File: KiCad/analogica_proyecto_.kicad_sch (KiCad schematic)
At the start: 4 parts, among them U2 ACS714xLCTR-50A, U3 ACS714xLCTR-50A

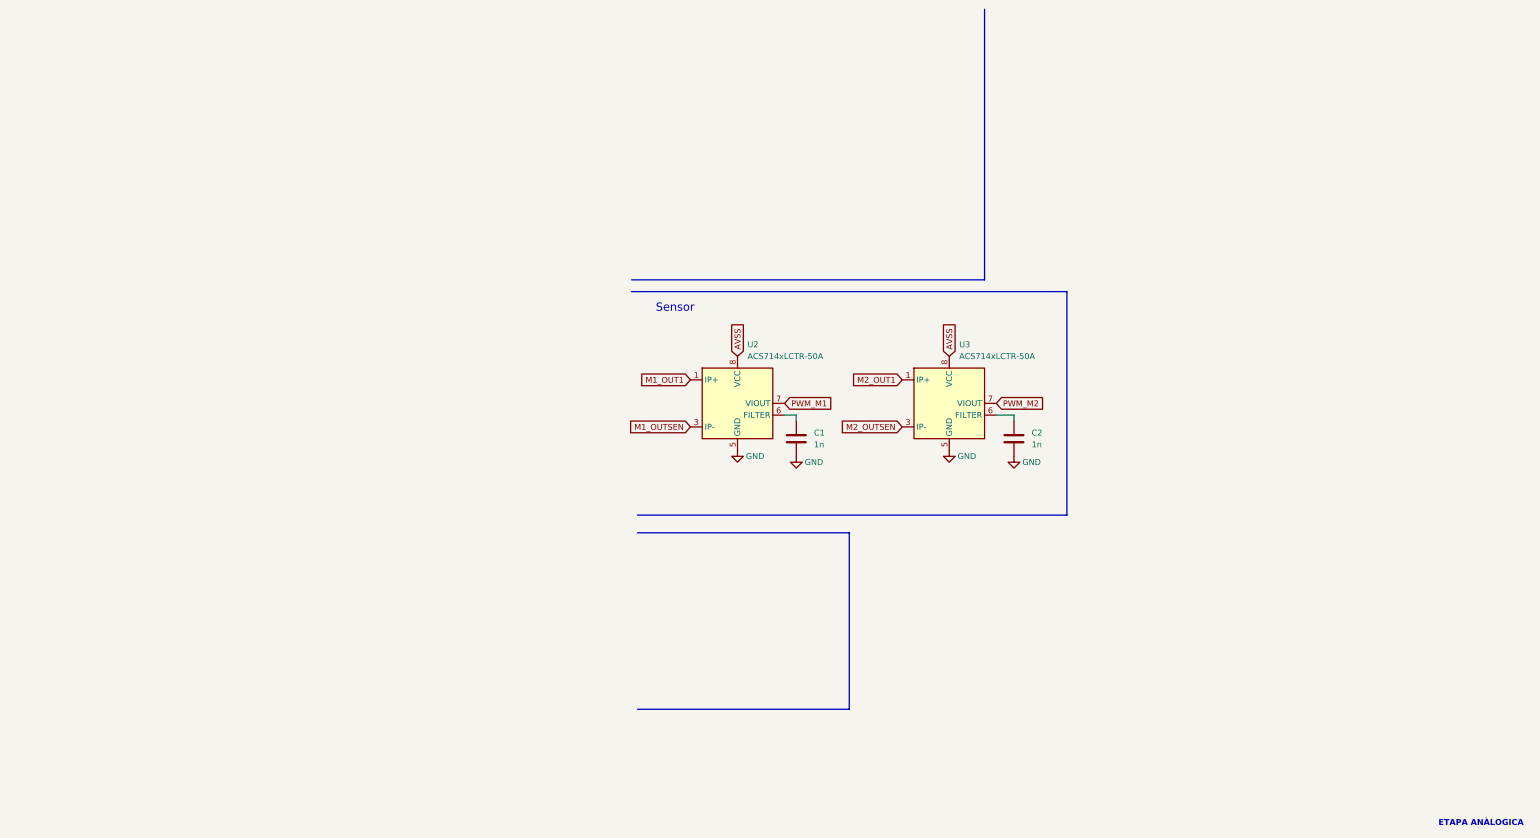
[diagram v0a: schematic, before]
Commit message: Nuevos cambios esquemativo v3
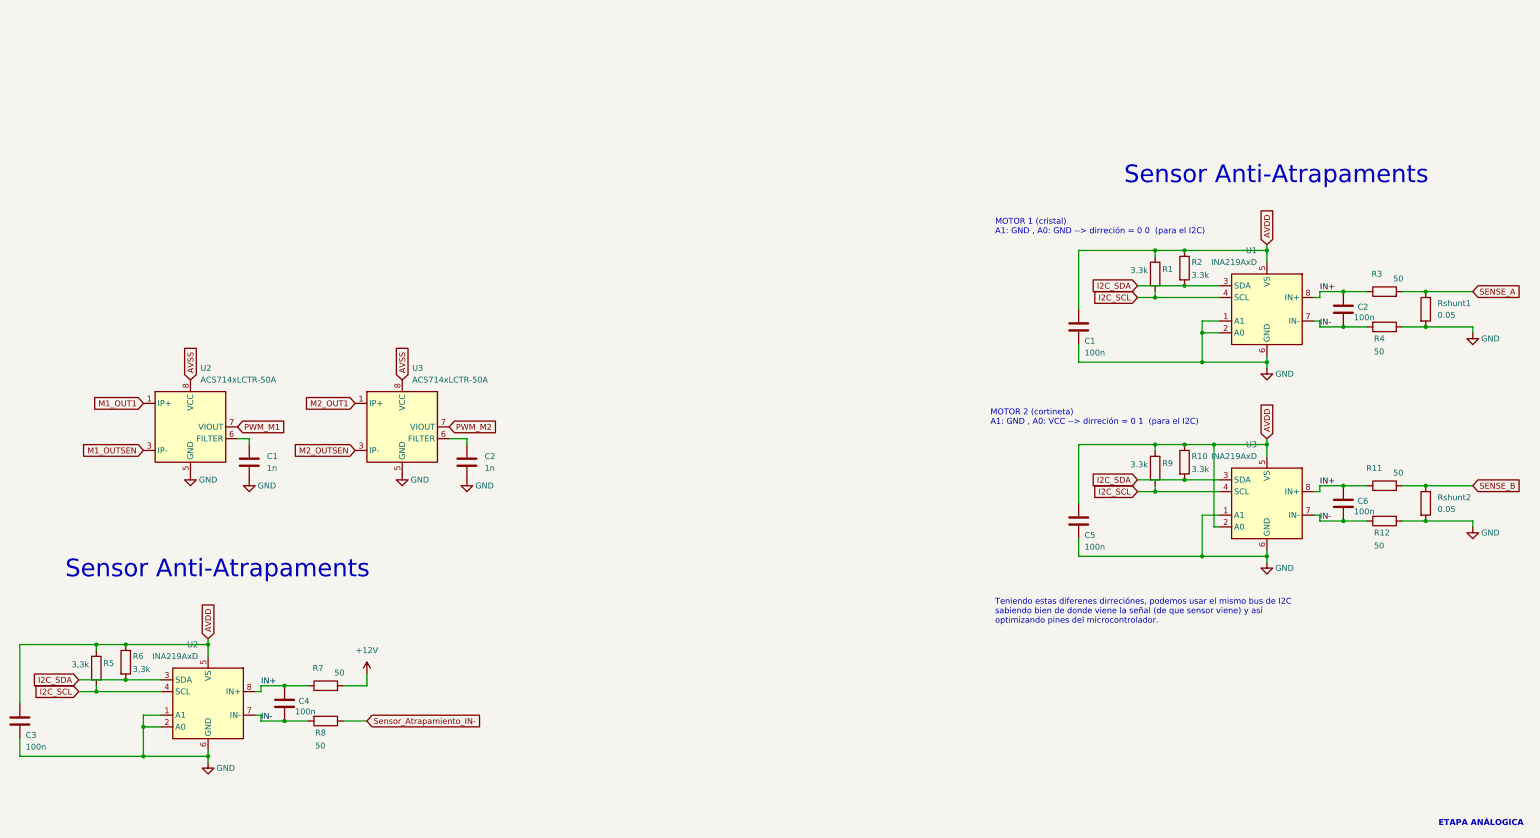
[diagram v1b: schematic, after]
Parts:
- added C1, C2, C3, C4, C5, C6: 100n, symbol Device:C
- added R1, R10, R2, R9: 3.3k, symbol Device:R
- added R11, R12, R3, R4, R7, R8: 50, symbol Device:R
- added R5, R6: 3,3k, symbol Device:R
- added Rshunt1, Rshunt2: 0.05, symbol Device:R
- added U1, U2, U3: INA219AxD, Package_SO:SOIC-8_3.9x4.9mm_P1.27mm, symbol Sensor_Energy:INA219AxD
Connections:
- net GND: now also C1.2, C3.2, C5.2, R12.1, R4.1, Rshunt1.2, Rshunt2.2, U1.1 (A1), U1.2 (A0), U1.6 (GND), U2.1 (A1), U2.2 (A0), U2.6 (GND), U3.1 (A1), U3.6 (GND)
- new net +12V: R7.2
- new net AVDD: C1.1, C3.1, C5.1, R1.1, R10.1, R2.1, R5.1, R6.1, R9.1, U1.5 (VS), U2.5 (VS), U3.2 (A0), U3.5 (VS)
- new net I2C_SCL: R1.2, R5.2, R9.2, U1.4 (SCL), U2.4 (SCL), U3.4 (SCL)
- new net I2C_SDA: R10.2, R2.2, R6.2, U1.3 (SDA), U2.3 (SDA), U3.3 (SDA)
- new net IN+: C2.1, C4.1, C6.1, R11.1, R3.1, R7.1, U1.8 (IN+), U2.8 (IN+), U3.8 (IN+)
- new net IN-: C2.2, C4.2, C6.2, R12.2, R4.2, R8.2, U1.7 (IN-), U2.7 (IN-), U3.7 (IN-)
- new net SENSE_A: R3.2, Rshunt1.1
- new net SENSE_B: R11.2, Rshunt2.1
- new net Sensor_Atrapamiento_IN-: R8.1
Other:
- note added: "MOTOR 1 (cristal) A1: GND , A0: GND --> dirreción = 0 0 (para el I2C)"
- note added: "MOTOR 2 (cortineta) A1: GND , A0: VCC --> dirreción = 0 1 (para el I2C)"
- note added: "Sensor Anti-Atrapaments"
- note added: "Teniendo estas diferenes dirreciónes, podemos usar el mismo bus de I2C sabiendo bien de donde viene la señal (de que sensor viene) y así optimizando pines del microcontrolador."
- note removed: "Sensor"
- moved on the sheet: C1, C2, U2, U3
